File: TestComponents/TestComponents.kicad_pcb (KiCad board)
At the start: 2 copper layers, 101.6 x 73.7 mm, 123 parts, among them J2-1 Conn_01x04_Male, J2-2 Conn_01x04_Male, J3V1 Conn_01x01_Male, J5 RFShield_OnePiece, J6 RFShield_OnePiece, SW1 SW_DPDT, SW2 SW_DP3T, SW3 SW_DPDT, U1 AD7991, U13 X, U2 ADS1219, U3 REF200AU, U4 MCP6L01x-xLT, U8 ADR510, U9 LM4040B

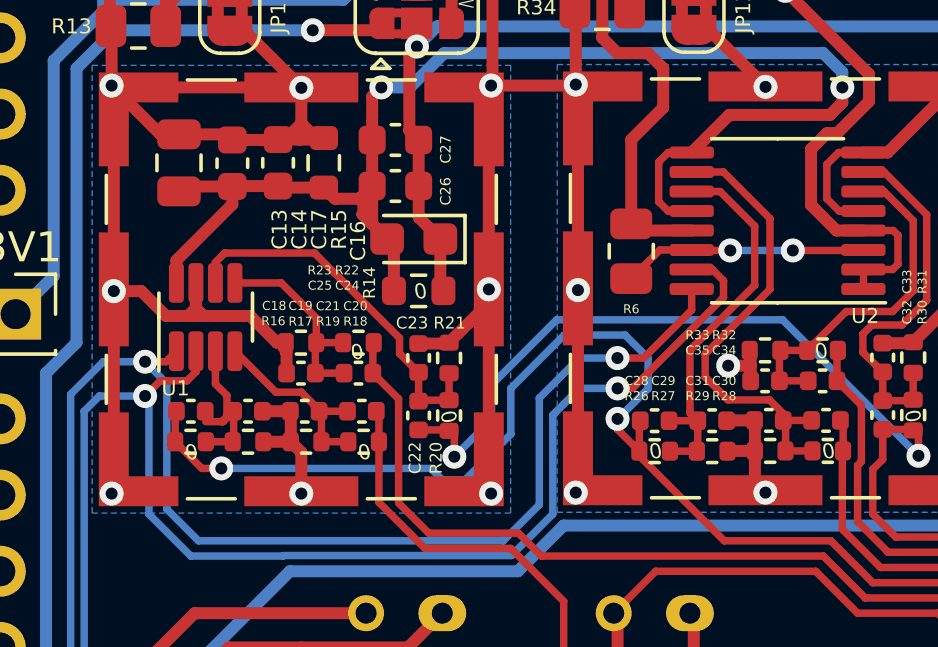
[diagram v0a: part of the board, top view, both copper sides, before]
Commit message: SpectDrone Development
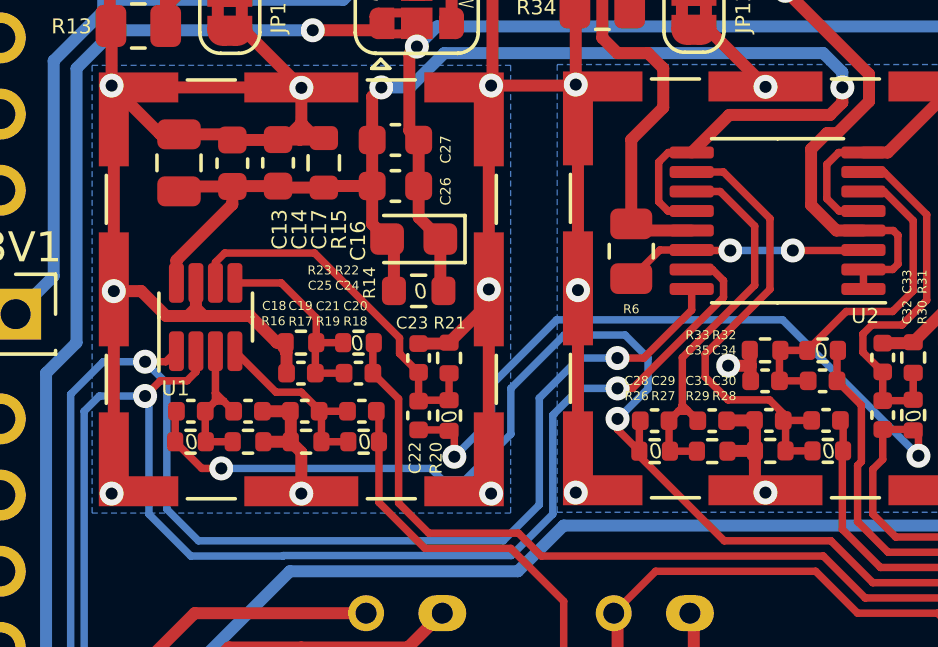
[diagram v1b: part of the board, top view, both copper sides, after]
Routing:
- net V_{RF}: track 45.7 -> 44.4 mm
- net S2_{RF}: track 5.85 -> 5.20 mm
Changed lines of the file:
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@@
     (effects (font (size 0.5 0.5) (thickness 0.075)))
   )
-  (gr_text "0" (at 139.6891 95.0566 180) (layer "F.SilkS")
+  (gr_text "0" (at 139.6891 94.7166 180) (layer "F.SilkS")
     (effects (font (size 0.5 0.5) (thickness 0.1) italic) (justify mirror))
   )
@@
     (effects (font (size 0.5 0.5) (thickness 0.125)))
   )
-  (gr_text "0" (at 145.2751 91.7546) (layer "F.SilkS")
+  (gr_text "0" (at 145.2751 91.4654) (layer "F.SilkS")
     (effects (font (size 0.5 0.5) (thickness 0.1) italic) (justify mirror))
   )
@@
     (effects (font (size 1 1) (thickness 0.15)) (justify left))
   )
-  (gr_text "0" (at 145.4529 95.0566 180) (layer "F.SilkS")
+  (gr_text "0" (at 145.4603 94.7166 180) (layer "F.SilkS")
     (effects (font (size 0.5 0.5) (thickness 0.1) italic) (justify mirror))
   )
@@
     (effects (font (size 1 1) (thickness 0.15)) (justify right))
   )
+  (segment (start 145.7447 86.2174) (end 144.1849 86.2174) (width 0.4) (layer "F.Cu") (net 1))
+  (segment (start 146.4697 88.2138) (end 146.4697 89.7131) (width 0.4) (layer "F.Cu") (net 1))
   (segment (start 161.417 82.931) (end 161.417 83.439) (width 0.4) (layer "F.Cu") (net 1))
   (segment (start 142.6581 86.2702) (end 142.6081 86.2202) (width 0.4) (layer "F.Cu") (net 1))
-  (segment (start 146.2418 87.9859) (end 145.4158 87.1599) (width 0.4) (layer "F.Cu") (net 1))
   (segment (start 141.0971 86.2202) (end 141.0841 86.2332) (width 0.4) (layer "F.Cu") (net 1))
-  (segment (start 145.4529 86.7762) (end 145.4529 87.1228) (width 0.4) (layer "F.Cu") (net 1))
-  (segment (start 144.5046 86.6427) (end 144.1321 86.2702) (width 0.4) (layer "F.Cu") (net 1))
   (segment (start 155.2956 86.741) (end 155.6056 87.051) (width 0.25) (layer "F.Cu") (net 1))
   (segment (start 142.6081 86.2202) (end 141.0971 86.2202) (width 0.4) (layer "F.Cu") (net 1))
   (segment (start 144.1321 86.2702) (end 142.6581 86.2702) (width 0.4) (layer "F.Cu") (net 1))
-  (segment (start 145.3194 86.6427) (end 145.4529 86.7762) (width 0.4) (layer "F.Cu") (net 1))
-  (segment (start 146.4697 88.2138) (end 146.4697 89.7131) (width 0.4) (layer "F.Cu") (net 1))
   (segment (start 156.3955 85.101) (end 155.6148 85.101) (width 0.25) (layer "F.Cu") (net 1))
+  (segment (start 146.2418 87.9859) (end 145.7447 87.4888) (width 0.4) (layer "F.Cu") (net 1))
   (segment (start 155.6056 87.051) (end 156.3955 87.051) (width 0.25) (layer "F.Cu") (net 1))
-  (segment (start 145.4529 87.1228) (end 145.4158 87.1599) (width 0.4) (layer "F.Cu") (net 1))
   (segment (start 145.7447 87.4888) (end 145.7447 86.2174) (width 0.4) (layer "F.Cu") (net 1))
   (segment (start 139.2201 88.694417) (end 139.2201 89.4487) (width 0.4) (layer "F.Cu") (net 1))
   (segment (start 141.0841 86.830417) (end 139.2201 88.694417) (width 0.4) (layer "F.Cu") (net 1))
+  (segment (start 144.1849 86.2174) (end 144.1321 86.2702) (width 0.4) (layer "F.Cu") (net 1))
   (segment (start 139.4681 86.2332) (end 139.3061 86.3952) (width 0.4) (layer "F.Cu") (net 1))
   (segment (start 141.0841 86.2332) (end 141.0841 86.830417) (width 0.4) (layer "F.Cu") (net 1))
   (segment (start 157.647889 83.848611) (end 156.3955 85.101) (width 0.4) (layer "F.Cu") (net 1))
+  (segment (start 146.2418 87.9859) (end 146.4697 88.2138) (width 0.4) (layer "F.Cu") (net 1))
   (segment (start 145.7447 84.6839) (end 145.7447 83.2363) (width 0.4) (layer "F.Cu") (net 1))
   (segment (start 161.007389 83.848611) (end 157.647889 83.848611) (width 0.4) (layer "F.Cu") (net 1))
   (segment (start 141.0841 86.2332) (end 139.4681 86.2332) (width 0.4) (layer "F.Cu") (net 1))
   (segment (start 161.417 83.439) (end 161.007389 83.848611) (width 0.4) (layer "F.Cu") (net 1))
-  (segment (start 146.2418 87.9859) (end 146.4697 88.2138) (width 0.4) (layer "F.Cu") (net 1))
   (segment (start 155.6148 85.101) (end 155.2956 85.4202) (width 0.25) (layer "F.Cu") (net 1))
-  (segment (start 145.3194 86.6427) (end 145.7447 86.2174) (width 0.4) (layer "F.Cu") (net 1))
   (segment (start 155.2956 85.4202) (end 155.2956 86.741) (width 0.25) (layer "F.Cu") (net 1))
   (segment (start 145.7447 86.2174) (end 145.7447 84.6839) (width 0.4) (layer "F.Cu") (net 1))
-  (segment (start 145.3194 86.6427) (end 144.5046 86.6427) (width 0.4) (layer "F.Cu") (net 1))
   (segment (start 145.7447 83.2363) (end 146.05 82.931) (width 0.4) (layer "F.Cu") (net 1))
   (via (at 146.05 82.931) (size 0.8) (drill 0.4) (layers "F.Cu" "B.Cu") (net 1))
@@
   (segment (start 154.94 91.948) (end 154.94 92.972614) (width 0.25) (layer "B.Cu") (net 5))
   (segment (start 153.932614 93.98) (end 153.924 93.98) (width 0.25) (layer "B.Cu") (net 5))
-  (segment (start 140.7311 94.0734) (end 140.7797 94.0734) (width 0.25) (layer "F.Cu") (net 6))
-  (segment (start 141.1271 93.726) (end 141.028044 93.726) (width 0.25) (layer "F.Cu") (net 6))
-  (segment (start 140.903872 93.900628) (end 140.7311 94.0734) (width 0.25) (layer "F.Cu") (net 6))
-  (segment (start 140.5201 92.8162) (end 140.903872 93.199972) (width 0.25) (layer "F.Cu") (net 6))
-  (segment (start 140.7797 94.0734) (end 141.1271 93.726) (width 0.25) (layer "F.Cu") (net 6))
-  (segment (start 140.5201 91.7237) (end 140.5201 92.8162) (width 0.25) (layer "F.Cu") (net 6))
-  (segment (start 141.0971 94.742) (end 140.1991 94.742) (width 0.25) (layer "F.Cu") (net 6))
-  (segment (start 141.028044 93.726) (end 140.903872 93.850172) (width 0.25) (layer "F.Cu") (net 6))
-  (segment (start 141.1271 93.726) (end 141.1271 94.712) (width 0.25) (layer "F.Cu") (net 6))
-  (segment (start 140.1991 94.0734) (end 140.7311 94.0734) (width 0.25) (layer "F.Cu") (net 6))
-  (segment (start 141.1271 94.712) (end 141.0971 94.742) (width 0.25) (layer "F.Cu") (net 6))
-  (segment (start 140.903872 93.900628) (end 140.903872 93.199972) (width 0.25) (layer "F.Cu") (net 6))
+  (segment (start 140.1991 94.742) (end 141.0971 94.742) (width 0.25) (layer "F.Cu") (net 6))
+  (segment (start 140.18 93.726) (end 140.18 94.7229) (width 0.25) (layer "F.Cu") (net 6))
+  (segment (start 140.79455 93.39345) (end 141.1271 93.726) (width 0.25) (layer "F.Cu") (net 6))
+  (segment (start 140.787 93.3859) (end 140.79455 93.39345) (width 0.25) (layer "F.Cu") (net 6))
+  (segment (start 140.5201 93.119) (end 140.5201 93.3859) (width 0.25) (layer "F.Cu") (net 6))
+  (segment (start 140.5201 91.7237) (end 140.5201 93.119) (width 0.25) (layer "F.Cu") (net 6))
+  (segment (start 140.5201 93.3859) (end 140.18 93.726) (width 0.25) (layer "F.Cu") (net 6))
+  (segment (start 140.18 94.7229) (end 140.1991 94.742) (width 0.25) (layer "F.Cu") (net 6))
+  (segment (start 140.5201 93.3859) (end 140.787 93.3859) (width 0.25) (layer "F.Cu") (net 6))
+  (segment (start 140.5201 93.119) (end 140.79455 93.39345) (width 0.25) (layer "F.Cu") (net 6))
   (segment (start 163.1305 110.871) (end 163.1715 110.912) (width 0.4) (layer "F.Cu") (net 7))
   (segment (start 147.2947 86.2174) (end 147.2947 84.6839) (width 0.4) (layer "F.Cu") (net 7))
@@
   (segment (start 183.261 82.58502) (end 183.261 83.6695) (width 0.4) (layer "F.Cu") (net 63))
   (segment (start 181.991 82.58502) (end 183.261 82.58502) (width 0.4) (layer "F.Cu") (net 63))
-  (segment (start 155.6704 94.0405) (end 156.5984 94.0405) (width 0.25) (layer "F.Cu") (net 65))
+  (segment (start 156.083 91.937079) (end 158.496 89.524079) (width 0.25) (layer "F.Cu") (net 65))
+  (segment (start 156.5984 94.0405) (end 156.24695 93.68905) (width 0.25) (layer "F.Cu") (net 65))
+  (segment (start 155.6704 95.0565) (end 156.5684 95.0565) (width 0.25) (layer "F.Cu") (net 65))
+  (segment (start 156.083 93.5979) (end 155.95545 93.72545) (width 0.25) (layer "F.Cu") (net 65))
+  (segment (start 156.083 93.5251) (end 156.083 91.937079) (width 0.25) (layer "F.Cu") (net 65))
+  (segment (start 155.6404 94.0405) (end 155.6404 95.0265) (width 0.25) (layer "F.Cu") (net 65))
+  (segment (start 156.083 93.5251) (end 156.083 93.5979) (width 0.25) (layer "F.Cu") (net 65))
+  (segment (start 158.496 87.5538) (end 157.3432 86.401) (width 0.25) (layer "F.Cu") (net 65))
+  (segment (start 157.3432 86.401) (end 156.3955 86.401) (width 0.25) (layer "F.Cu") (net 65))
+  (segment (start 156.24695 93.68905) (end 156.083 93.5251) (width 0.25) (layer "F.Cu") (net 65))
+  (segment (start 155.95545 93.72545) (end 155.6404 94.0405) (width 0.25) (layer "F.Cu") (net 65))
+  (segment (start 155.95545 93.72545) (end 156.21055 93.72545) (width 0.25) (layer "F.Cu") (net 65))
+  (segment (start 155.6404 95.0265) (end 155.6704 95.0565) (width 0.25) (layer "F.Cu") (net 65))
   (segment (start 158.496 89.524079) (end 158.496 87.5538) (width 0.25) (layer "F.Cu") (net 65))
-  (segment (start 156.5684 95.0565) (end 155.6704 95.0565) (width 0.25) (layer "F.Cu") (net 65))
-  (segment (start 158.496 87.5538) (end 157.3432 86.401) (width 0.25) (layer "F.Cu") (net 65))
-  (segment (start 156.5984 94.0405) (end 156.5984 95.0265) (width 0.25) (layer "F.Cu") (net 65))
-  (segment (start 156.5984 94.0405) (end 156.337 93.7791) (width 0.25) (layer "F.Cu") (net 65))
-  (segment (start 156.5984 95.0265) (end 156.5684 95.0565) (width 0.25) (layer "F.Cu") (net 65))
-  (segment (start 156.337 93.7791) (end 156.337 91.683079) (width 0.25) (layer "F.Cu") (net 65))
-  (segment (start 157.3432 86.401) (end 156.3955 86.401) (width 0.25) (layer "F.Cu") (net 65))
-  (segment (start 156.337 91.683079) (end 158.496 89.524079) (width 0.25) (layer "F.Cu") (net 65))
+  (segment (start 156.21055 93.72545) (end 156.24695 93.68905) (width 0.25) (layer "F.Cu") (net 65))
   (segment (start 157.4552 85.751) (end 159.004 87.2998) (width 0.25) (layer "F.Cu") (net 66))
   (segment (start 159.5256 95.0469) (end 160.4236 95.0469) (width 0.25) (layer "F.Cu") (net 66))
